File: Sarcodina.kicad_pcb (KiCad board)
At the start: 2 copper layers, 94 x 94 mm, 375 parts, among them SW7 SW_PUSH

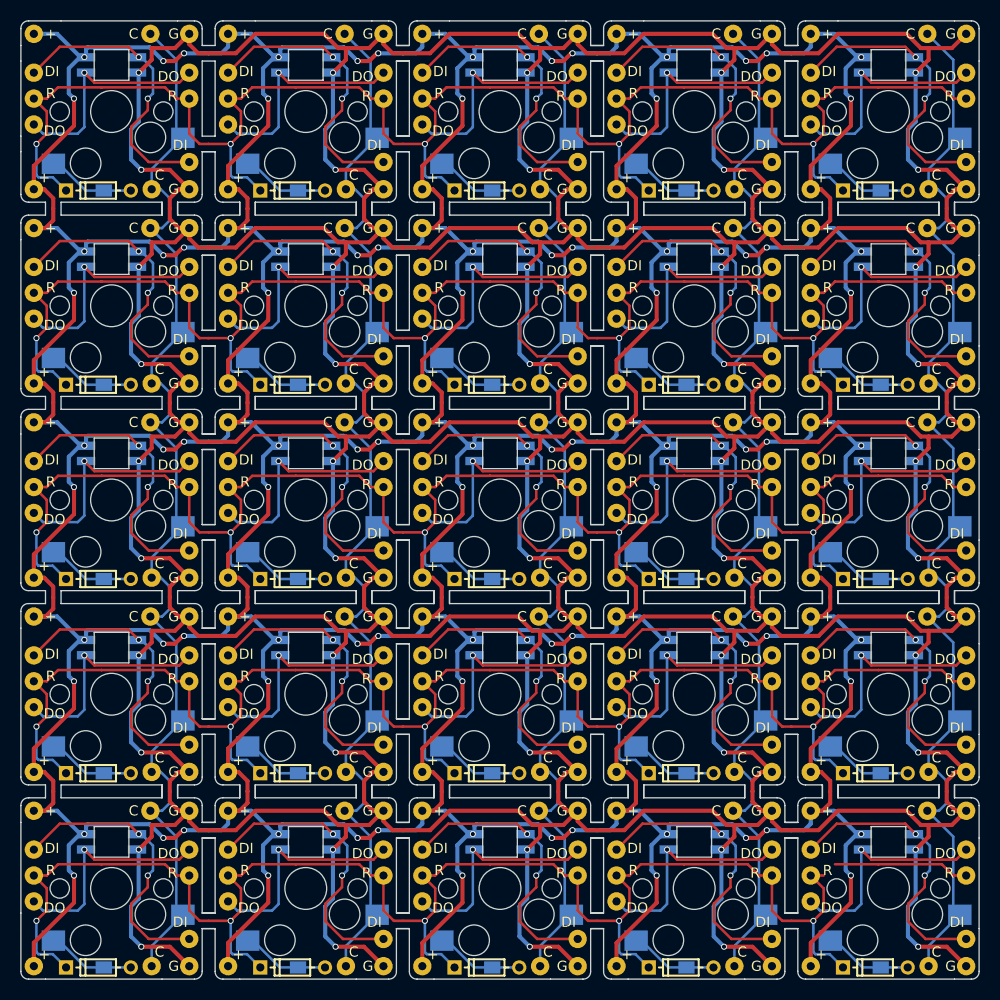
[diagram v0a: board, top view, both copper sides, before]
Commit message: Fixed edges.
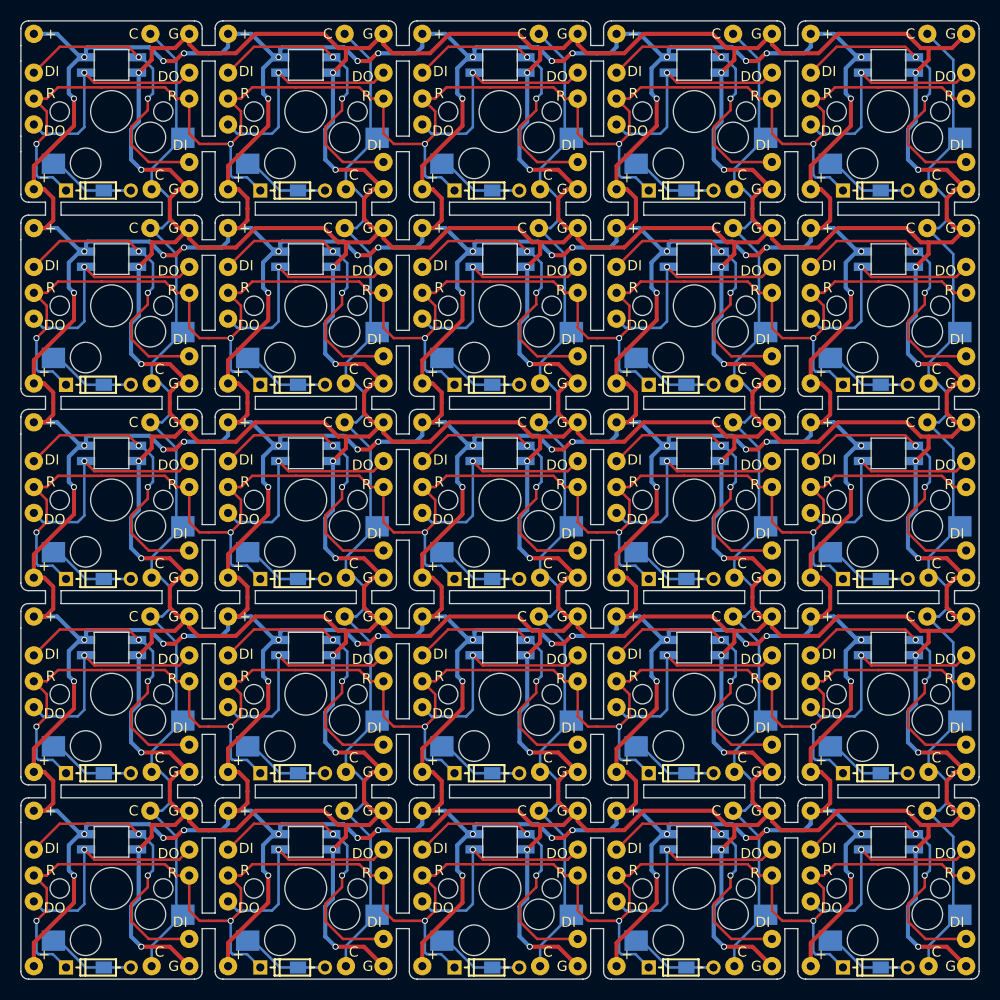
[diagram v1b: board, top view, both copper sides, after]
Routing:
- net row4: track 170.8 -> 172.4 mm
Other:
- outline, holes or cut-outs redrawn
